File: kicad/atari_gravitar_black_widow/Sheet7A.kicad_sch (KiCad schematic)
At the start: 27 parts

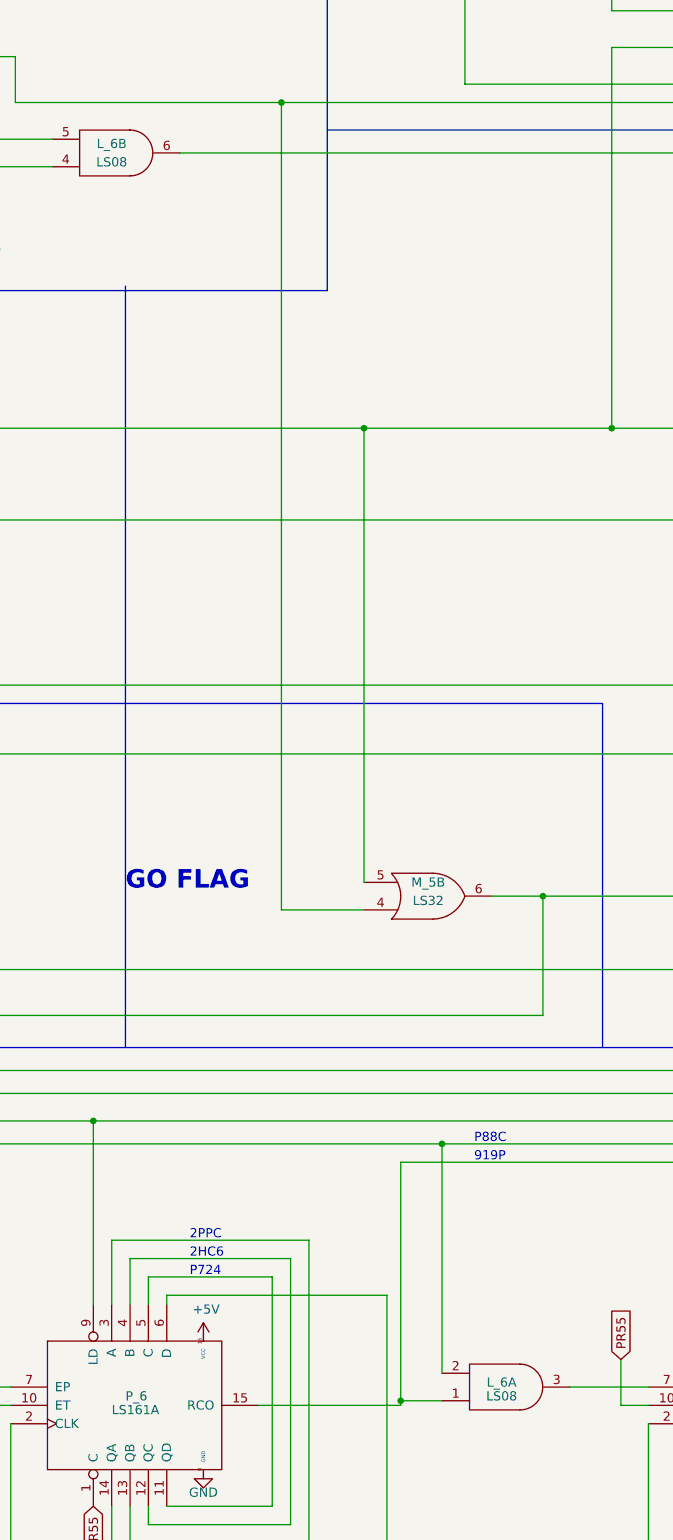
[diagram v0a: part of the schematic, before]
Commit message: 4A DONE
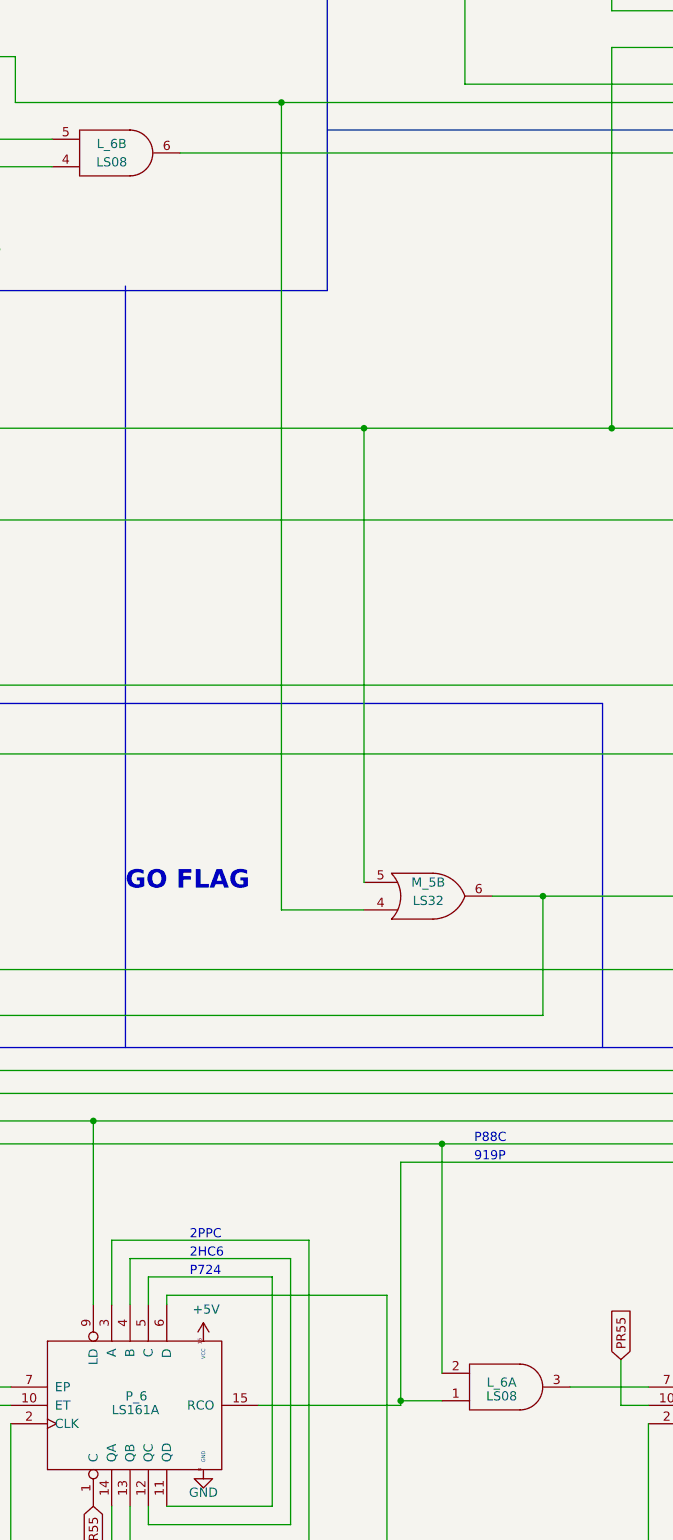
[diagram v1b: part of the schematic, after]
